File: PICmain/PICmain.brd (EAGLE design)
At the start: 100 x 75 mm, 20 parts, among them IC2 74HC00N, J1 PIC_ICSP_6_PIN, M1 MOTORSHORT, M2 MOTORSHORT, U1 PIC16F1778

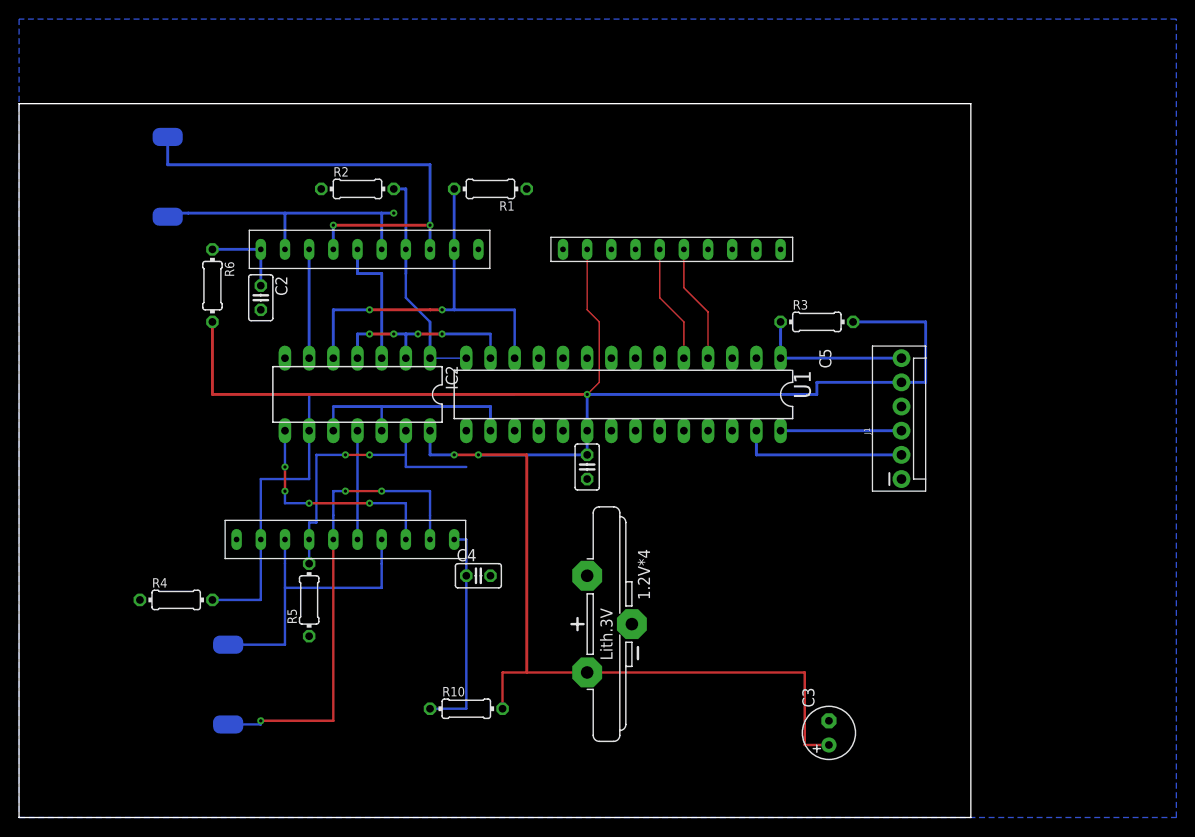
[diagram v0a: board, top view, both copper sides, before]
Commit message: update mcc
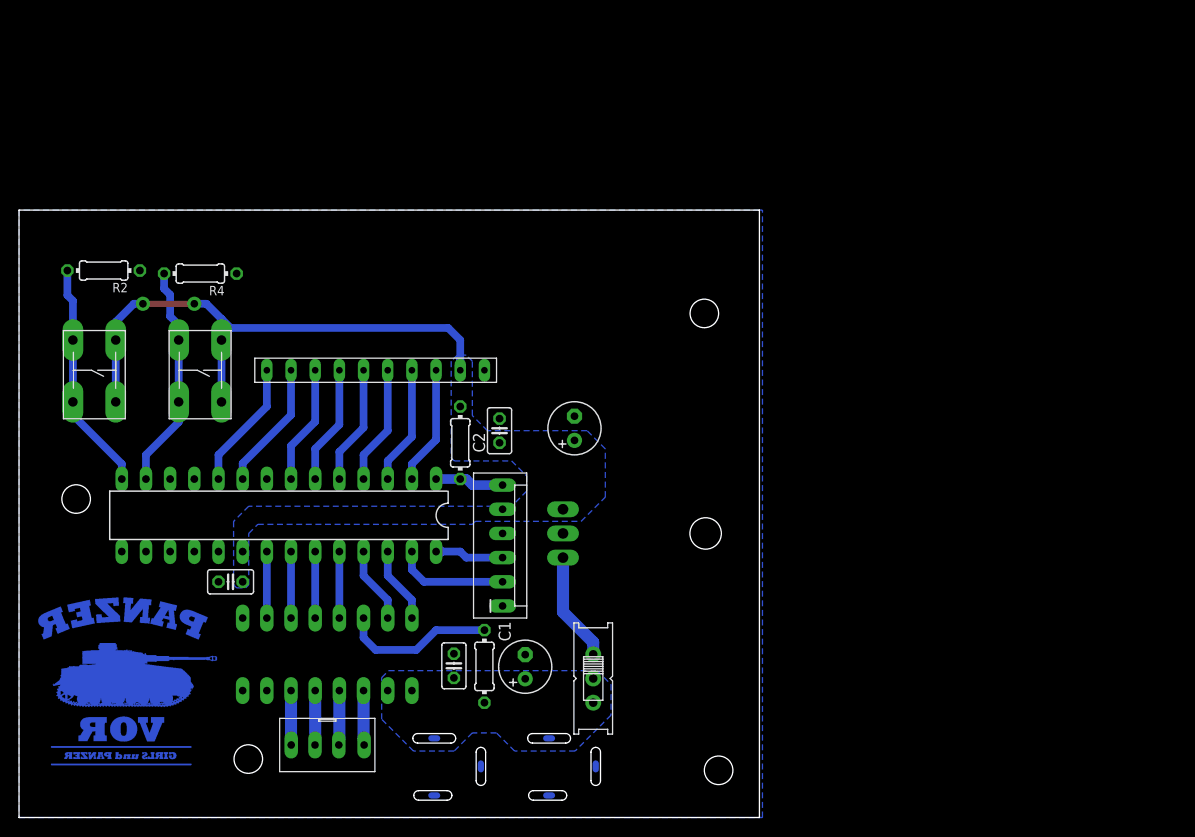
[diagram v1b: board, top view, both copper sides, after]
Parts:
- removed 1.2V*4: CR2430V, battery:CR2430V
- removed M1, M2: MOTORSHORT, SparkFun-Electromechanical:VIBE-MOTOR-10MM-SMD
- removed R10, R6: 10, rcl:0204/7
- removed R5: 10k, rcl:0204/7
- removed U$3: AE-NJL5901AR-8CH, AE-NJL5901AR-8CH:AE-NJL5901AR-8CH
- added C1: 100u, rcl:E2,5-6
- added CONNECTOR1, CONNECTOR2: TACT_SWITCH, akizuki:TACT_SWITCH
- added S1: (no value), adafruit:EG1218
- added U$1: AE-TC78H653FTG, akizuki:AE-TC78H653FTG
- added U$5: MJ-179PH, akizuki:MJ-179PH
- added U$6: AE-NJL5901AR-8CH, akizuki:AE-NJL5901AR-8CH
- C2: value (none) -> 104
- IC2: value 74HC00N -> 7805T; device 74xx-eu:DIL14 -> adafruit (2):TO220H
- R1, R2, R4: value 10k -> (none)
- U$2: value MP4212 -> 4PIN; device MP4212:MP4212 -> con-ei:4PIN
- U$4: value MP4212 -> MJ-179PH; device MP4212:MP4212 -> akizuki:MJ-179PH
- moved U$2 52.3 mm to (32.4, 7.62)
- moved R1 50.2 mm to (48.9, 15.9), turned to 270 degrees
- moved J1 44.0 mm to (50.8, 22.2)
- moved C3 41.7 mm to (58.4, 40.9)
- moved R3 39.6 mm to (46.4, 39.4), turned to 90 degrees
- moved C5 39.4 mm to (22.2, 24.8), turned to 180 degrees
- moved U1 38.4 mm to (27.3, 31.8)
- moved IC2 34.9 mm to (67.3, 29.8), flipped to the bottom, turned to 90 degrees
- moved R4 34.4 mm to (19.1, 57.1), turned to 180 degrees
- moved C2 28.7 mm to (50.5, 40.6), turned to 90 degrees
- moved R2 28.0 mm to (8.89, 57.5), turned to 180 degrees
- moved U$4 27.8 mm to (48.5, 5.37), turned to 90 degrees
- moved C4 9.80 mm to (45.7, 15.9), turned to 90 degrees
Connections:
- removed net CCP1: IC2.2, IC2.4, U1.13
- removed net CCP2: IC2.10, IC2.12, U1.16
- removed net DVDD1: C2.1, R6.1, U$2.S34
- removed net DVDD3: C4.1, R10.1, U$4.S34
- removed net SEL11: IC2.5, R1.2, U$2.G1, U1.12
- removed net SEL12: IC2.1, R2.2, U$2.G2, U1.14
- removed net SEL21: IC2.9, R4.2, U$4.G1, U1.15
- removed net SEL22: IC2.13, R5.2, U$4.G2, U1.17
- new net DVDD: C1.+, C4.1, R1.2, S1.P, S1.S, U$1.VM@0, U$1.VM@1, U$4.J, U$5.J
- new net IN1: U$1.IN1, U1.22
- new net IN2: U$1.IN2, U1.21
- new net IN3: U$1.IN3, U1.23
- new net IN4: U$1.IN4, U1.24
- new net LARGE: U$1.LARGE, U1.26
- new net MODE: U$1.MODE, U1.25
- new net N$12: CONNECTOR2.2@0, CONNECTOR2.2@1, R2.2, U1.14
- new net N$13: U$1.OUT3, U$2.P$3
- new net N$14: U$1.OUT4, U$2.P$4
- new net N$15: U$1.OUT2, U$2.P$1
- new net N$16: R1.1, U$1.STBY
- new net N$17: IC2.1, S1.O
- net GND: now also C1.-, IC2.2, U$1.GND@0, U$1.GND@1, U$1.GND@2, U$4.B, U$4.S, U$5.B, U$5.S, U$6.GND; no longer 1.2V*4.-, IC2.7, R1.1, R5.1, U$2.S12, U$3.GND, U$4.S12
- net N$1: now also U$1.OUT1, U$2.P$2; no longer M2.+, U$4.D1, U$4.D3
- net N$10: now also U$6.OUT6, U1.7; no longer M1.-, U$2.D2, U$2.D4
- net N$11: now also U$6.OUT8, U1.10; no longer IC2.6, U$2.G4
- net N$18: now also U$6.OUT7, U1.9; no longer U$3.OUT3, U1.5
- net N$19: now also CONNECTOR1.2@0, CONNECTOR1.2@1, R4.2, U1.13; no longer U$3.OUT4, U1.4
- net N$2: now also U$6.OUT1, U1.2; no longer M2.-, U$4.D2, U$4.D4
- net N$4: now also U$6.OUT2, U1.3; no longer IC2.8, U$4.G4
- net N$6: now also U$6.OUT3, U1.4; no longer IC2.3, U$2.G3
- net N$8: now also U$6.OUT4, U1.5; no longer IC2.11, U$4.G3
- net N$9: now also U$6.OUT5, U1.6; no longer M1.+, U$2.D1, U$2.D3
- net VCC: now also C2.1, CONNECTOR1.1@0, CONNECTOR1.1@1, CONNECTOR2.1@0, CONNECTOR2.1@1, IC2.3, U$6.VIN; no longer 1.2V*4.+, IC2.14, R10.2, R6.2, U$3.VIN
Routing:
- net VCC: track 213.1 -> 62.6 mm, vias 3 -> 2
- net SEL21: track 53.3 -> 0.00 mm
- net SEL11: track 41.9 -> 0.00 mm, vias 2 -> 0
- net N$9: track 52.1 -> 12.5 mm, vias 2 -> 0
- net N$2: track 50.8 -> 12.5 mm, vias 3 -> 0
- net SEL22: track 31.8 -> 0.00 mm, vias 2 -> 0
- net N$1: track 32.3 -> 5.72 mm
- net N$12: track 0.00 -> 24.3 mm
- net CCP2: track 24.1 -> 0.00 mm
- net SEL12: track 23.9 -> 0.00 mm
- net DVDD3: track 22.9 -> 0.00 mm
- net CCP1: track 21.6 -> 0.00 mm, vias 4 -> 0
- net N$10: track 31.8 -> 12.5 mm, vias 1 -> 0
- net N$16: track 0.00 -> 16.2 mm
- net N$4: track 24.1 -> 12.5 mm, vias 4 -> 0
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- added copper zone on layer 16, net DVDD
- added copper zone on layer 16, net VCC
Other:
- board size 100 x 75 mm -> 77.8 x 63.8 mm
